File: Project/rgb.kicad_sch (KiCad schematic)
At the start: 33 parts, among them U5 74AHCT1G125

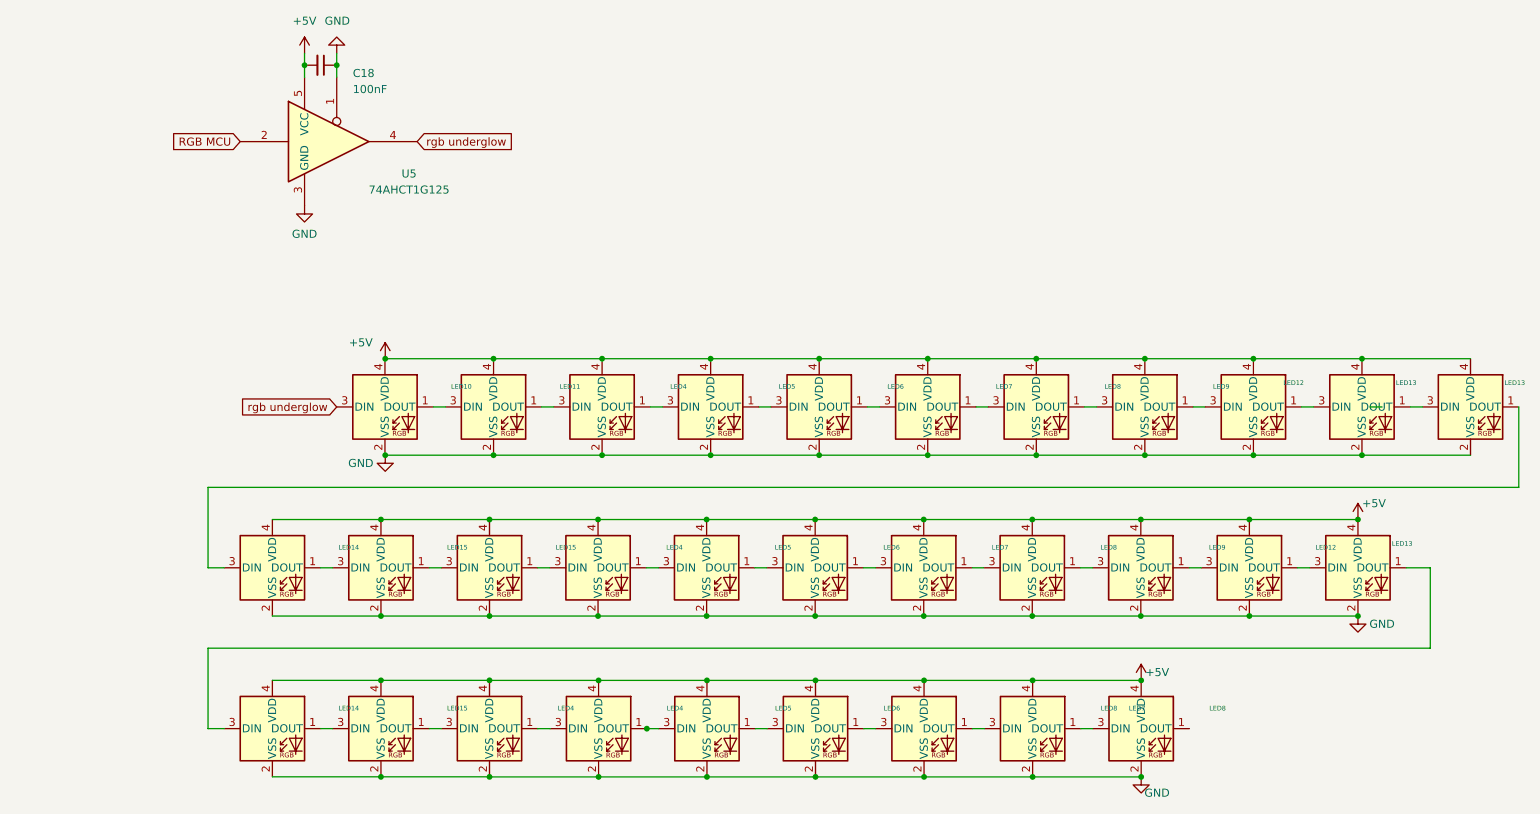
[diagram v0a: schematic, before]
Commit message: new bottom row, proto project created, rgb revised
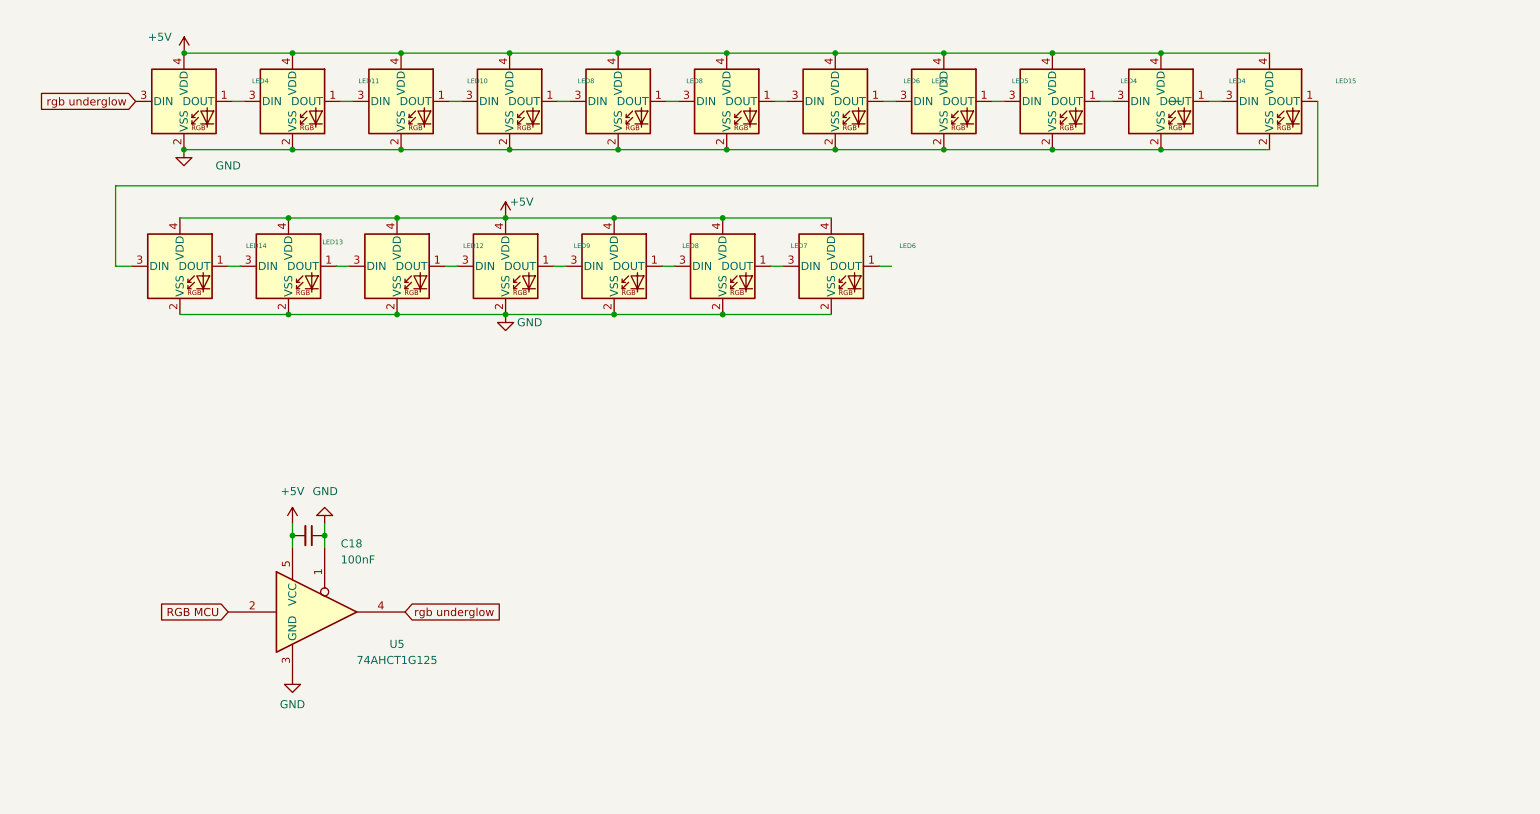
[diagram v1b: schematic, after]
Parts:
- removed LED12, LED13 (x2), LED14, LED15 (x2), LED4, LED5 (x2), LED6, LED7, LED8, LED9: WS2812_2020, PCM_marbastlib-various:LED_WS2812_2020, symbol PCM_marbastlib-various:WS2812_2020
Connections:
- net rgb underglow: now also LED4.3 (DIN); no longer LED10.3 (DIN)
- net at LED6.1 (DOUT): no longer LED7.3 (DIN)
- net at LED6.3 (DIN): now also LED7.1 (DOUT)
- net at LED12.1 (DOUT): now also LED9.3 (DIN); no longer LED13.3 (DIN)
- net at LED12.3 (DIN): now also LED13.1 (DOUT); no longer LED9.1 (DOUT)
- net at LED15.1 (DOUT): now also LED14.3 (DIN); no longer LED4.3 (DIN)
- net at LED15.3 (DIN): now also LED4.1 (DOUT); no longer LED14.1 (DOUT)
- net at LED4.1 (DOUT): now also LED11.3 (DIN)
- net at LED11.1 (DOUT): now also LED10.3 (DIN); no longer LED4.3 (DIN)
- net at LED4.3 (DIN): now also LED5.1 (DOUT); no longer LED4.1 (DOUT)
- net at LED4.1 (DOUT): now also LED4.3 (DIN); no longer LED5.3 (DIN)
- net at LED10.1 (DOUT): now also LED8.3 (DIN); no longer LED11.3 (DIN)
- net at LED7.1 (DOUT): now also LED6.3 (DIN); no longer LED8.3 (DIN)
- net at LED7.3 (DIN): now also LED8.1 (DOUT); no longer LED6.1 (DOUT)
- net at LED8.1 (DOUT): now also LED8.3 (DIN)
- net at LED8.1 (DOUT): now also LED7.3 (DIN); no longer LED9.3 (DIN)
- net at LED8.3 (DIN): now also LED9.1 (DOUT); no longer LED7.1 (DOUT)
- new net: LED13.3 (DIN), LED14.1 (DOUT)
- new net: LED5.3 (DIN), LED6.1 (DOUT)
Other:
- moved on the sheet: C18, LED10, LED11, LED12, LED13, LED14, LED15, LED4, LED5, LED6, LED7, LED8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
